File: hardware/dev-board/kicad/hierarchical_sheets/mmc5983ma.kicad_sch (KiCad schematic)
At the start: 2 parts, among them U4 MMC5983MA

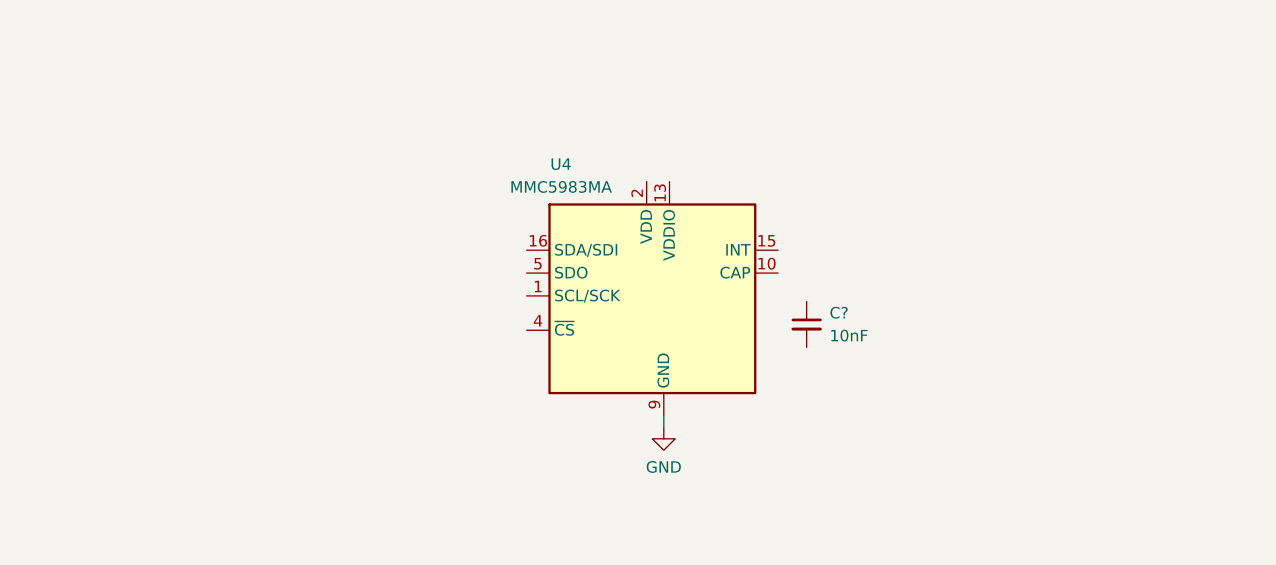
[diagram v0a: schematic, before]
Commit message: rf is hard
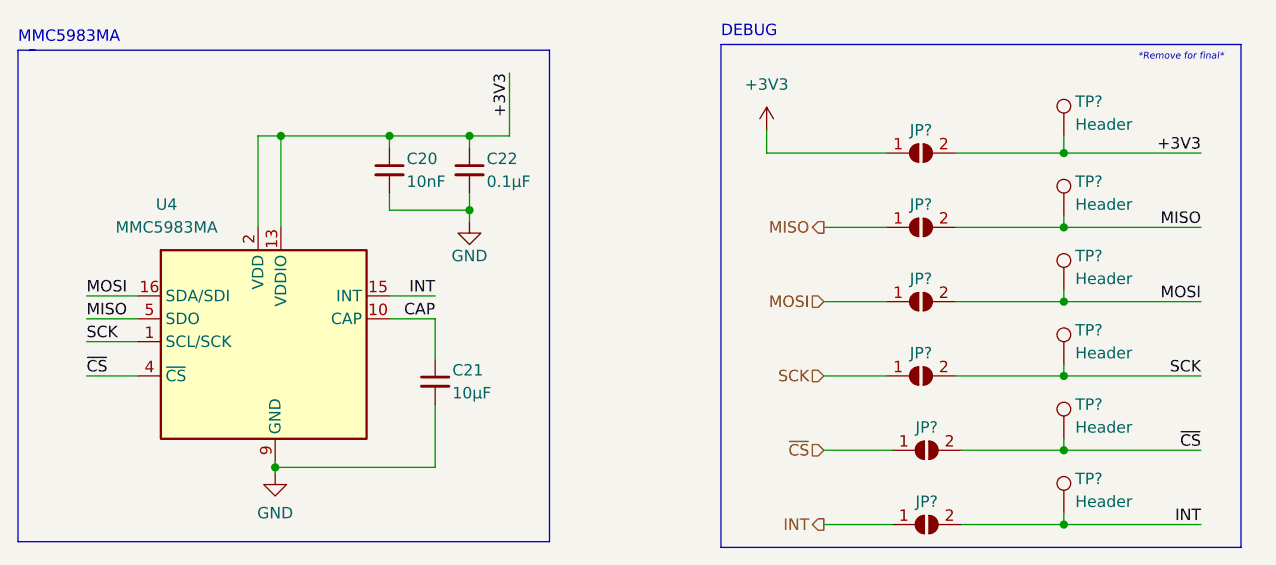
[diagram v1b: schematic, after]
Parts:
- added C20: 10nF, symbol Device:C_Small
- added C22: 0.1μF, symbol Device:C_Small
- added JP? (x6): SolderJumper_2_Open, Jumper:SolderJumper-2_P1.3mm_Open_RoundedPad1.0x1.5mm, symbol Jumper:SolderJumper_2_Open
- added TP? (x6): Header, Connector_PinHeader_2.54mm:PinHeader_1x01_P2.54mm_Vertical, symbol Connector:TestPoint
- C21: renamed from C?; value 10nF -> 10μF
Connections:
- net GND: now also C21.2, C20.2, C22.2
- net CAP: now reaches C21.1
- net CAP: now also U4.10 (CAP)
- net SCK: now reaches U4.1 (SCL/SCK)
- net SCK: now also JP?.1 (A), JP?.2 (B), TP?.1
- net +3V3: now reaches U4.13 (VDDIO)
- net +3V3: now also U4.2 (VDD), C20.1, C22.1, JP?.1 (A), JP?.2 (B), TP?.1
- net INT: now reaches U4.15 (INT)
- net INT: now also JP?.1 (A), JP?.2 (B), TP?.1
- net MOSI: now reaches U4.16 (SDA/SDI)
- net MOSI: now also JP?.1 (A), JP?.2 (B), TP?.1
- net ~{CS}: now reaches U4.4 (~{CS})
- net ~{CS}: now also JP?.1 (A), JP?.2 (B), TP?.1
- net MISO: now reaches U4.5 (SDO)
- net MISO: now also JP?.1 (A), JP?.2 (B), TP?.1
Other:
- note added: "*Remove for final*"
- note added: "DEBUG"
- note added: "MMC5983MA"
- moved on the sheet: C21, U4
